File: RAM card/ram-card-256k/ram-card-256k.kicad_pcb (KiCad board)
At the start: 2 copper layers, 41.9 x 53.3 mm, 12 parts, among them J1 RAM card connector, U1 HC138, U2 KM681000BLG, U3 KM681000BLG

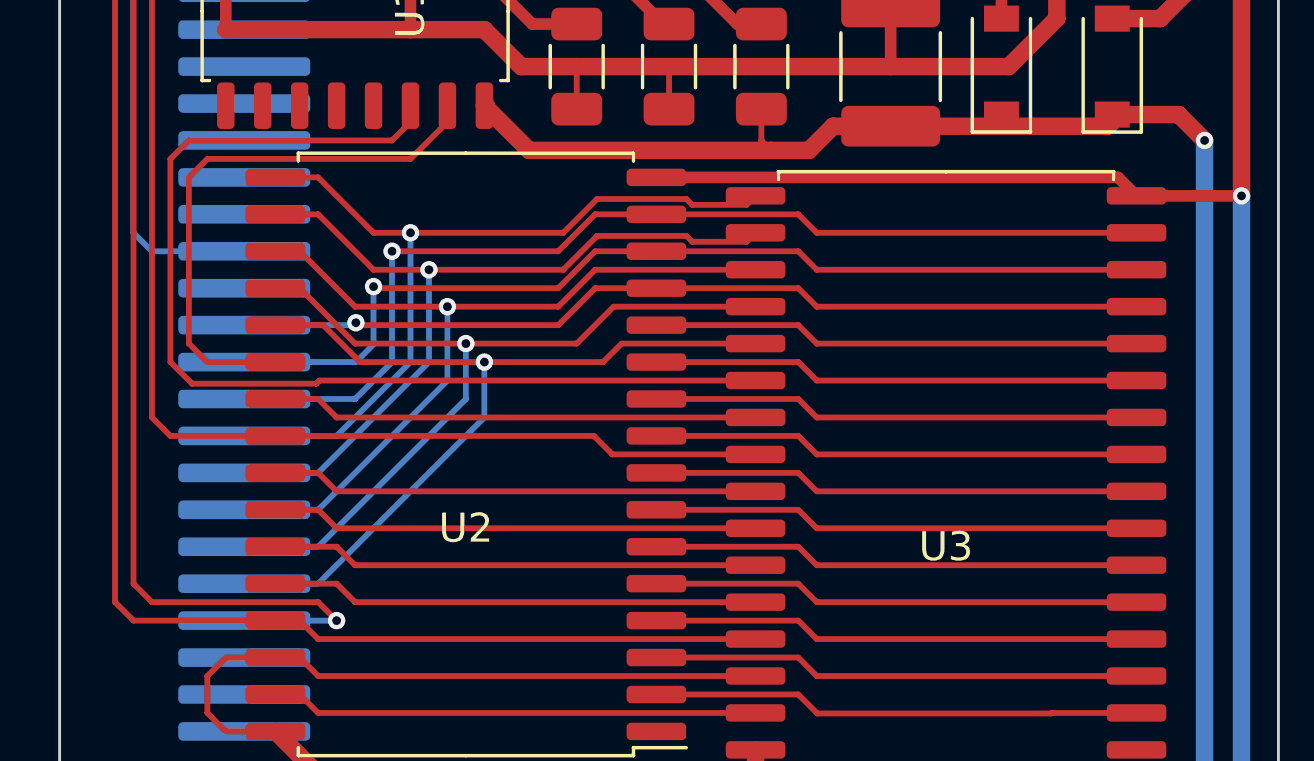
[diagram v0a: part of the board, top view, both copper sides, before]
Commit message: Data bus
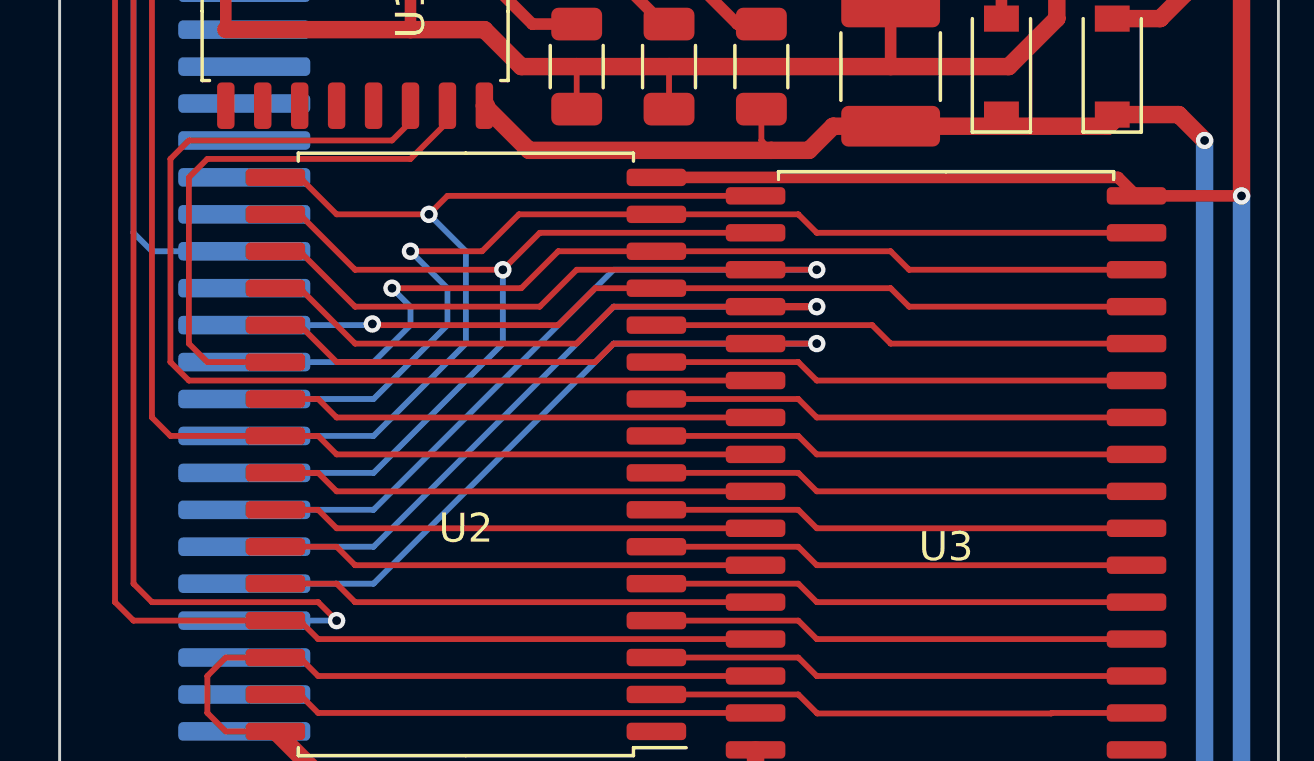
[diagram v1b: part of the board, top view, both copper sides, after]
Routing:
- net /D5: track 29.2 -> 43.0 mm
- net /D7: track 29.8 -> 42.5 mm
- net /D6: track 29.5 -> 40.8 mm
- net /D3: track 29.2 -> 31.2 mm
- net /D4: track 29.1 -> 31.1 mm
- net /D2: track 35.8 -> 36.9 mm
